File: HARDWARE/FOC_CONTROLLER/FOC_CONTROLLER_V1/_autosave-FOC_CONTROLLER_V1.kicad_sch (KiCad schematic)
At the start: 18 parts, among them IC1 STSPIN32G0A2

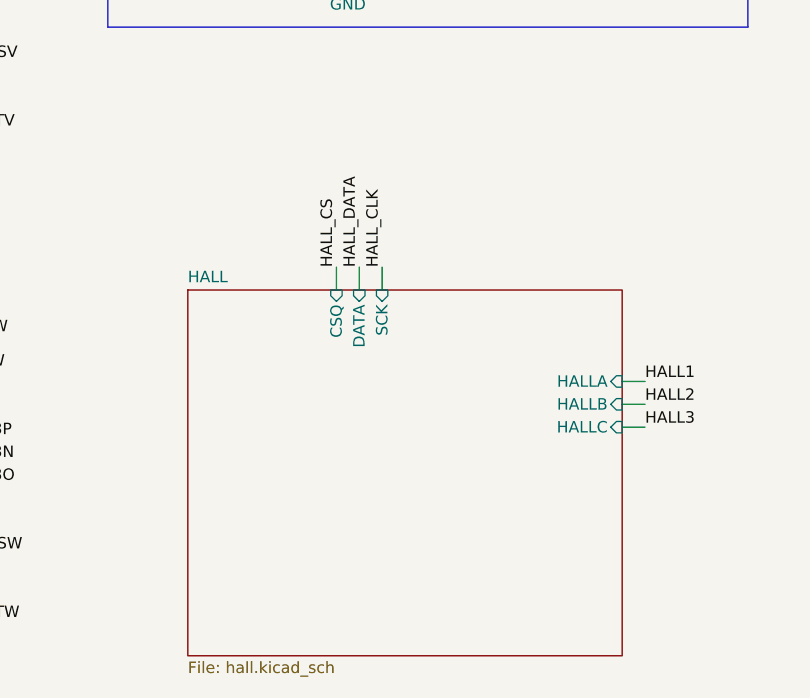
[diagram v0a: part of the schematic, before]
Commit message: up
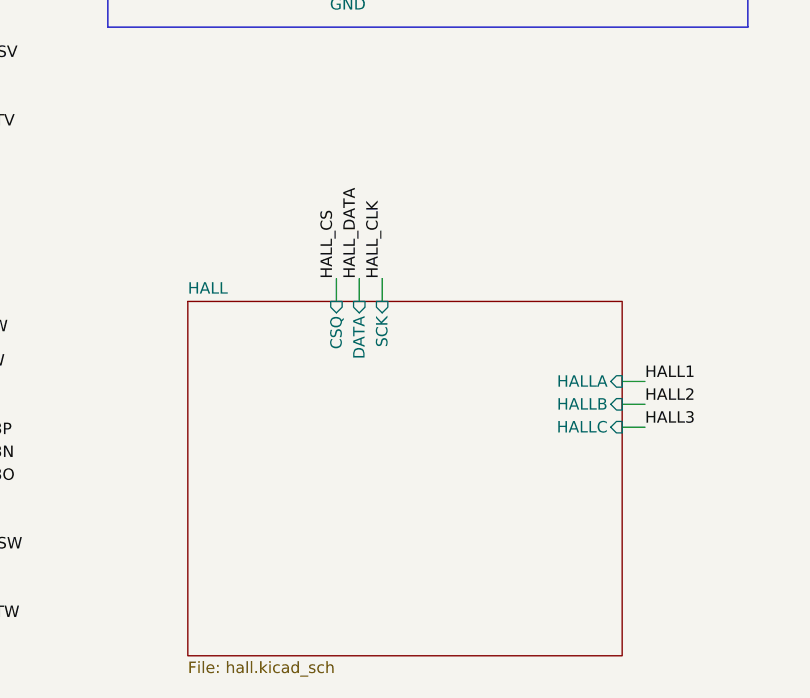
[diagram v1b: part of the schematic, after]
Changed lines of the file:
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@@
 	(wire
 		(pts
-			(xy 110.49 137.16) (xy 110.49 139.7)
+			(xy 110.49 138.43) (xy 110.49 140.97)
 		)
 		(stroke
@@
 	(wire
 		(pts
-			(xy 107.95 137.16) (xy 107.95 139.7)
+			(xy 107.95 138.43) (xy 107.95 140.97)
 		)
 		(stroke
@@
 	(wire
 		(pts
-			(xy 105.41 137.16) (xy 105.41 139.7)
+			(xy 105.41 138.43) (xy 105.41 140.97)
 		)
 		(stroke
@@
 	)
 	(label "HALL_CS"
-		(at 105.41 137.16 90)
+		(at 105.41 138.43 90)
 		(effects
 			(font
@@
 	)
 	(label "HALL_DATA"
-		(at 107.95 137.16 90)
+		(at 107.95 138.43 90)
 		(effects
 			(font
@@
 	)
 	(label "HALL_CLK"
-		(at 110.49 137.16 90)
+		(at 110.49 138.43 90)
 		(effects
 			(font
@@
 	)
 	(sheet
-		(at 88.9 139.7)
-		(size 48.26 40.64)
+		(at 88.9 140.97)
+		(size 48.26 39.37)
 		(exclude_from_sim no)
 		(in_bom yes)
@@
 		)
 		(property "Sheetname" "HALL"
-			(at 88.9 138.9884 0)
+			(at 88.9 140.2584 0)
 			(effects
 				(font
@@
 		)
 		(pin "CSQ" input
-			(at 105.41 139.7 90)
+			(at 105.41 140.97 90)
 			(effects
 				(font
@@
 		)
 		(pin "DATA" input
-			(at 107.95 139.7 90)
+			(at 107.95 140.97 90)
 			(effects
 				(font
@@
 		)
 		(pin "SCK" input
-			(at 110.49 139.7 90)
+			(at 110.49 140.97 90)
 			(effects
 				(font
